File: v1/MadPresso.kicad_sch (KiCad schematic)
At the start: 38 parts, among them J1 Conn_01x07, J2 Conn_01x03, Q1 2N7002, Q2 2N7002, Q3 BC847, U1 LTV-356T, U2 WeMos_D1_mini

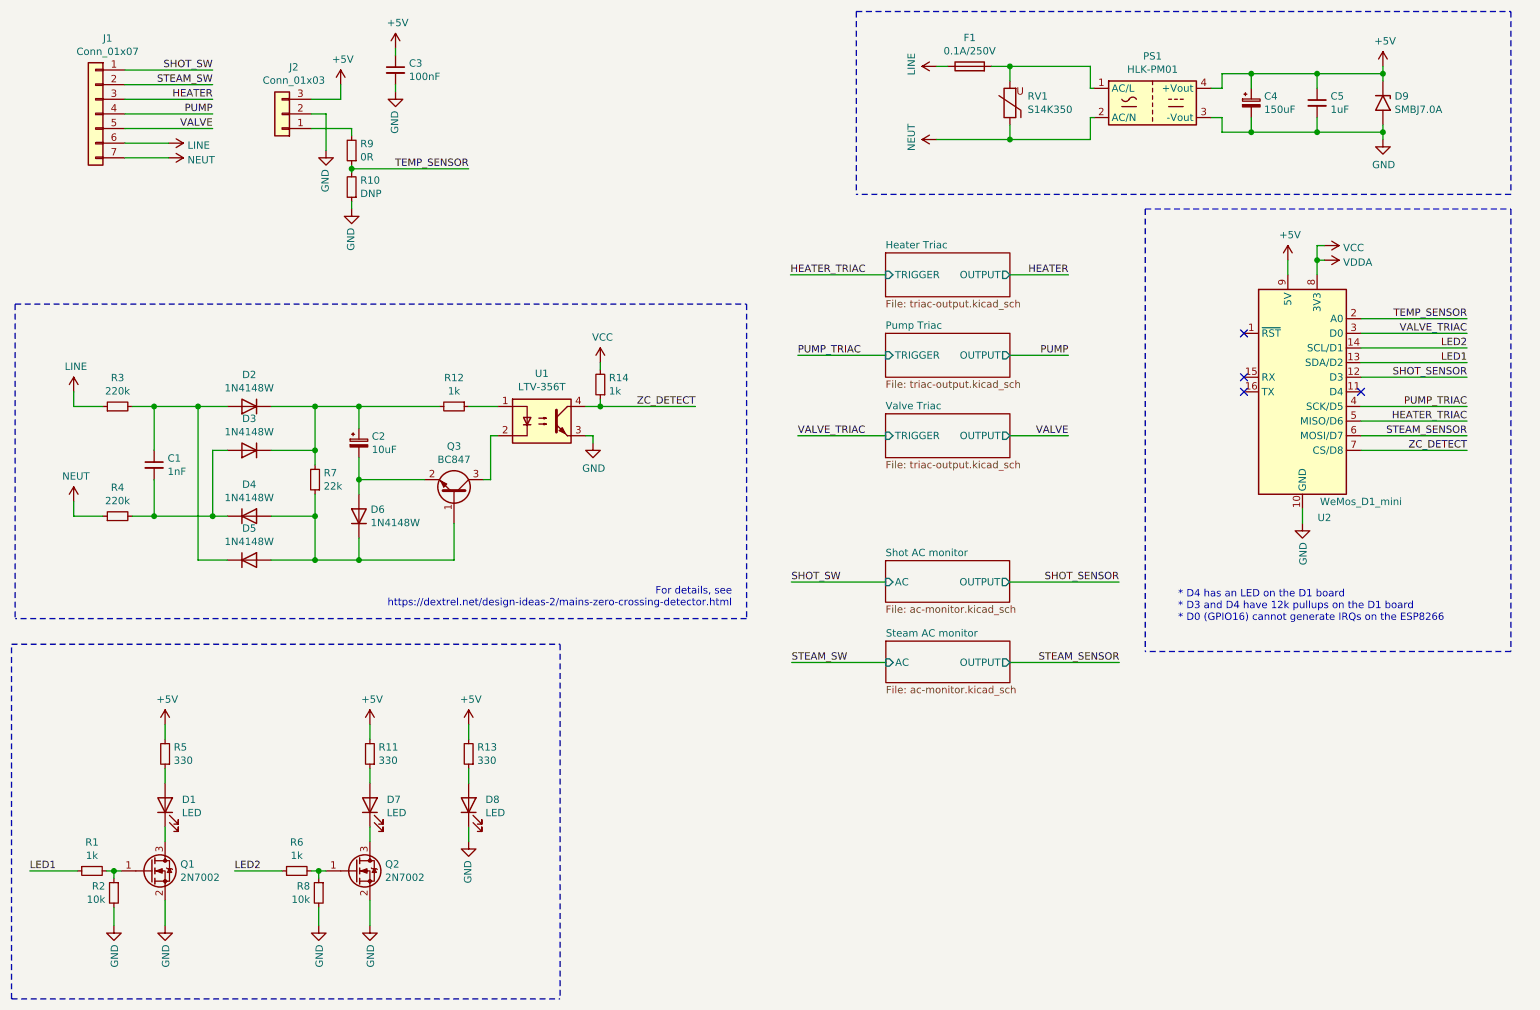
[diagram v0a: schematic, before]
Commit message: cleanups
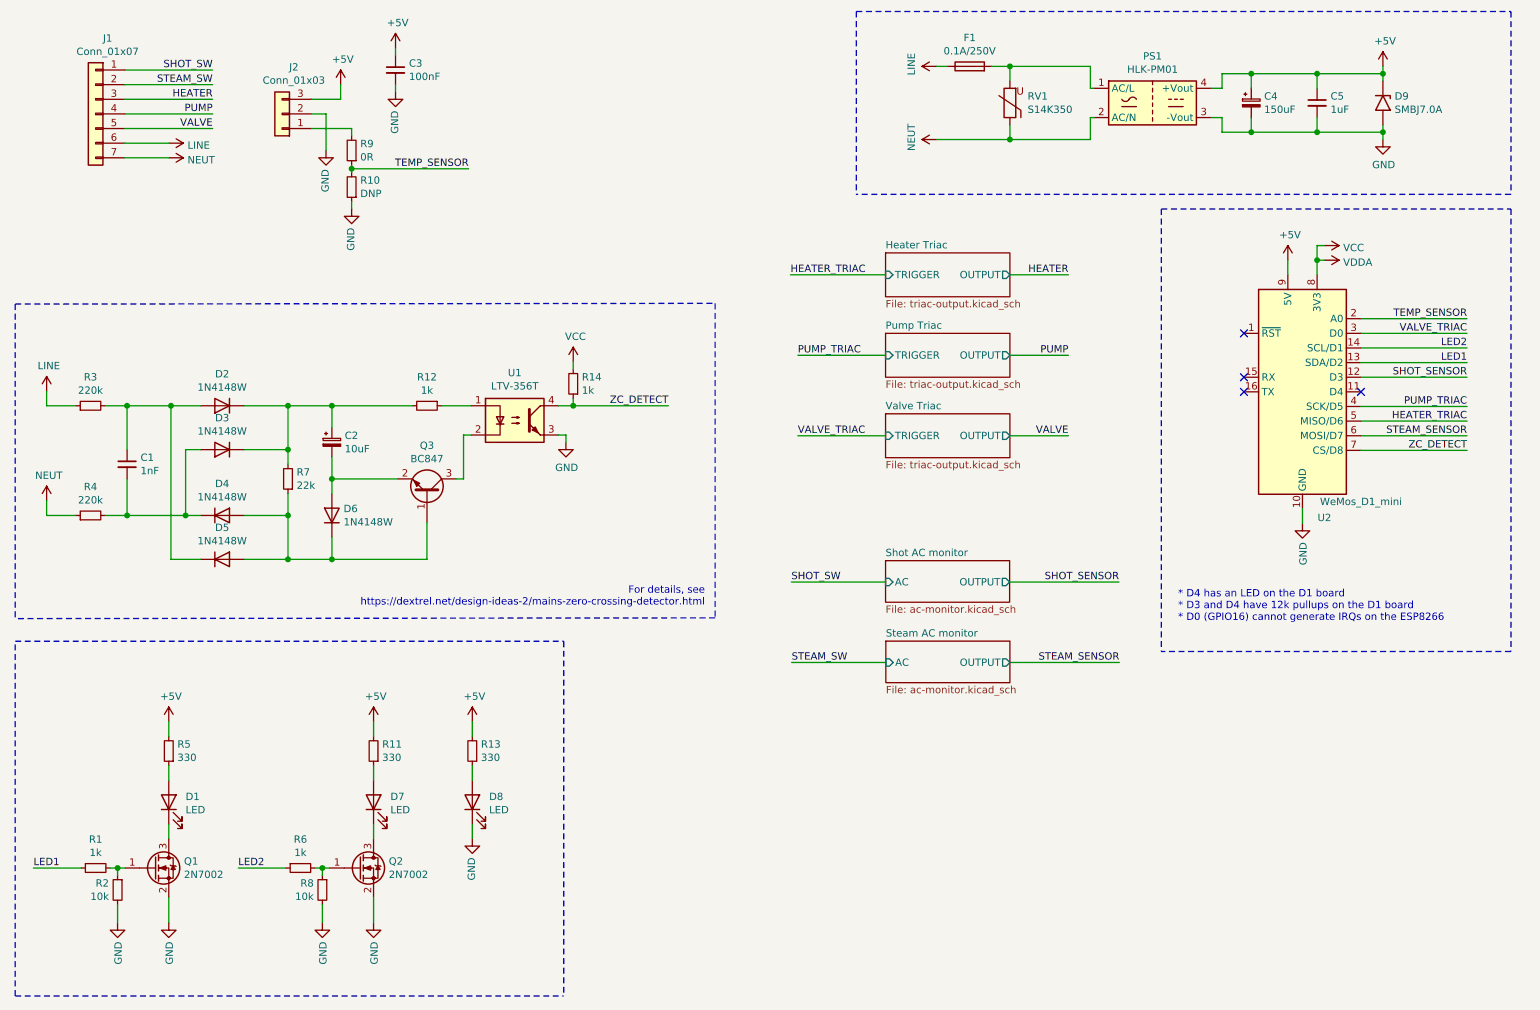
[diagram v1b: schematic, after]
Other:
- moved on the sheet: C1, C2, D1, D2, D3, D4, D5, D6, D7, D8, Q1, Q2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
